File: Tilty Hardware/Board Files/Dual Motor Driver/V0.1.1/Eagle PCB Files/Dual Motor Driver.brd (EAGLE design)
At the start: 50.8 x 50.8 mm, 31 parts, among them J1 AVR_SPI_PRG_6PTH, Q1 16MHz, U1 ATMEGA328P, U2 L298_BRIDGE_DRIVER, U3 LM2931

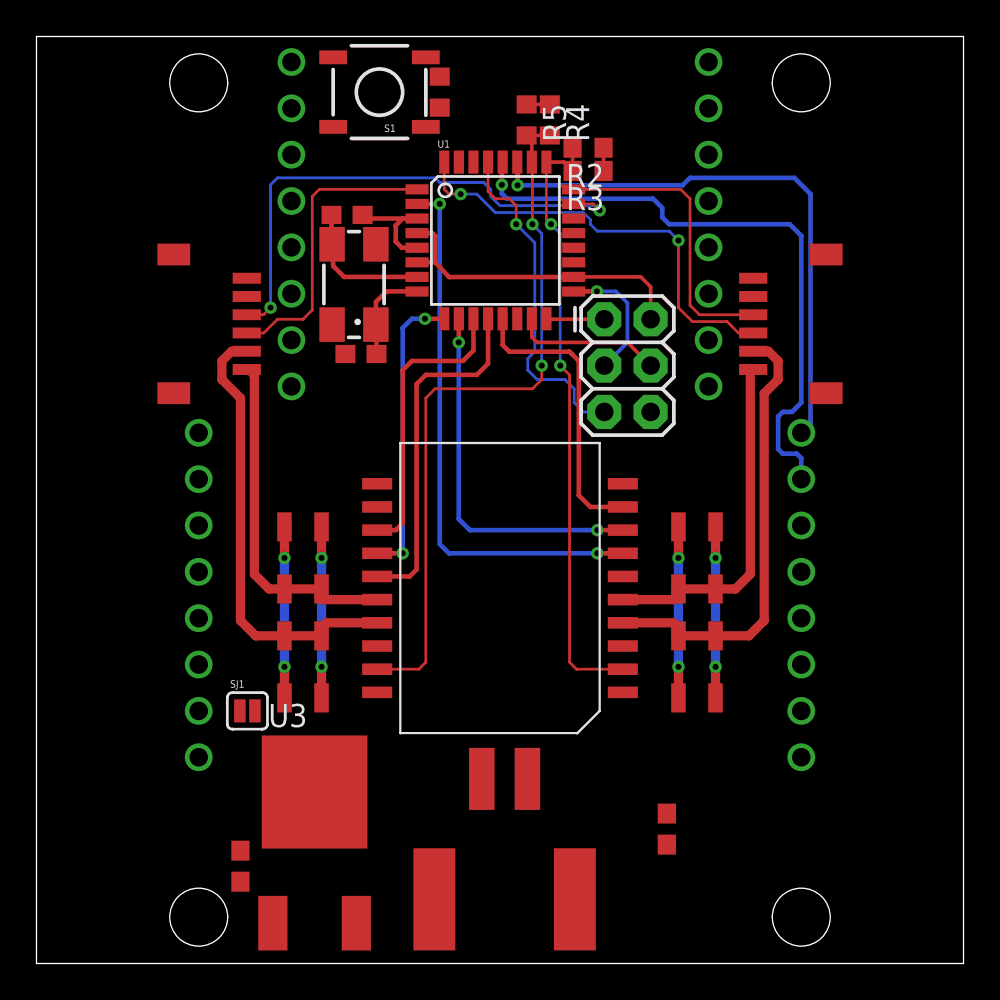
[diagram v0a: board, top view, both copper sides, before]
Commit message: Nearly finalized dual motor driver add-on
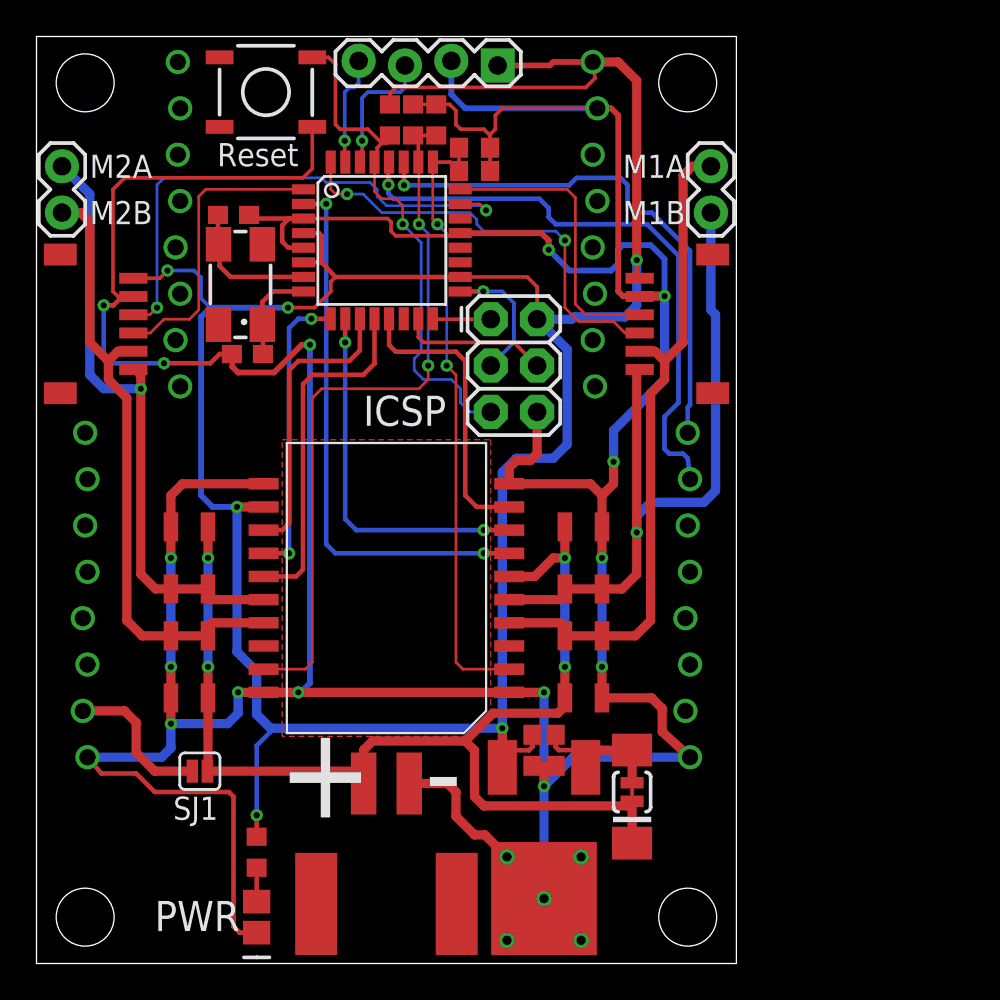
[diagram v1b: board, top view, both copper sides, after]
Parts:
- added D10: (no value), SparkFun-LED:LED-0805
- added D9: (no value), diode:DO214AA
- added JP10, JP9: (no value), SparkFun-Connectors:1X02
- added JP8: (no value), SparkFun-Connectors:1X04_LOCK
- added R6: (no value), resistor:R0603
- added SJ2: (no value), SparkFun-Passives:SJ_2S-TRACE
- JP1, JP2, JP3, JP4: value (none) -> 8-PIN_HEADER; device pinhead:1X08_NO_SS -> My Parts:8-PIN_RECEPTACLE_LOCK_NO-SS
- moved C7 18.4 mm to (28.4, 11.7), turned to 270 degrees
- moved U3 12.6 mm to (27.8, 6.35), turned to 180 degrees
- moved C6 8.54 mm to (27.2, 11.7), turned to 270 degrees
- moved JP7 6.48 mm to (19.2, 5.59)
- moved D7 6.22 mm to (29.0, 22.2)
- moved D8 6.22 mm to (29.0, 16.3)
- moved R4 6.22 mm to (21.9, 46.2)
- moved U1 6.22 mm to (18.9, 39.6)
- moved C2 6.22 mm to (11.6, 33.4)
- moved C8 6.22 mm to (10.8, 41.0)
- moved D3 6.22 mm to (7.37, 22.2)
- moved D4 6.22 mm to (7.37, 16.3)
- moved D5 6.22 mm to (9.40, 16.3)
- moved D6 6.22 mm to (9.40, 22.2)
- moved JP1 6.22 mm to (7.75, 40.5)
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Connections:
- new net N$1: D10.1, R6.2
- new net N$3: C7.1, D9.A, SJ2.1, U3.P$2
- new net RX: JP8.3, U1.30
- new net TX: JP8.4, U1.31
- net +24V: now also D9.C, SJ2.2; no longer C7.1, U3.P$2
- net +5V: now also JP4.P$1, JP8.1, R6.1; no longer JP4.1
- net GND: now also D10.2, JP2.P$1, JP3.P$1, JP4.P$2, JP8.2, U2.20; no longer JP2.1, JP3.1, JP4.2
- net M1A: now also JP9.2
- net M1B: now also JP9.1
- net M2A: now also JP10.2
- net M2B: now also JP10.1
- net N$5: now also JP2.P$2; no longer JP2.2
- net SCL: now also JP3.P$7; no longer JP3.7
- net SDA: now also JP3.P$8; no longer JP3.8
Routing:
- net GND: track 27.1 -> 276.5 mm, vias 4 -> 20
- net +5V: track 17.7 -> 148.8 mm, vias 0 -> 6
- net +24V: track 18.7 -> 63.7 mm
- net M1B: track 19.1 -> 40.2 mm, vias 0 -> 1
- net M2A: track 19.2 -> 34.4 mm, vias 0 -> 1
- net M1A: track 24.8 -> 37.1 mm
- net M2B: track 24.6 -> 34.4 mm
- net RESET: track 18.7 -> 28.3 mm
- net N$5: track 0.00 -> 8.34 mm
- net N$3: track 0.00 -> 7.67 mm
- net RX: track 0.00 -> 7.36 mm, vias 0 -> 1
- net TX: track 0.00 -> 6.03 mm, vias 0 -> 1
- net N$1: track 0.00 -> 1.86 mm
- net SDA: track 31.2 -> 29.4 mm
- net SCL: track 34.5 -> 32.9 mm
- added copper zone on layer 1, net GND
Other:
- board size 50.8 x 50.8 mm -> 38.4 x 50.8 mm
- board text added: "+"
- board text added: "-"
- board text added: "5v"
- board text added: "Driver Add-on"
- board text added: "Dual Motor"
- board text added: "GND"
- board text added: "ICSP"
- board text added: "IMU"
- board text added: "M1A"
- board text added: "M1B"
- board text added: "M2A"
- board text added: "M2B"
- board text added: "PWR"
- board text added: "Reset"
- board text added: "Rx"
- board text added: "SJ1"
- board text added: "Tx"
